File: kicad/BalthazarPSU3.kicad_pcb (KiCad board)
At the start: 2 copper layers, 85.9 x 25.4 mm, 84 parts, among them IC1 BQ24193, J1 AudioIN, J2 USB_C_Receptacle_USB2.0, J3 5-15V / 3-5A, J4 AudioOUT, J7 uC host, J8 5V 3A, J9 12V 2A, Q1 IRF7404, Q2 BSS138, Q3 BSS138, U1 PAM8403-SOP16, U3 TPS63020, U4 LM2623

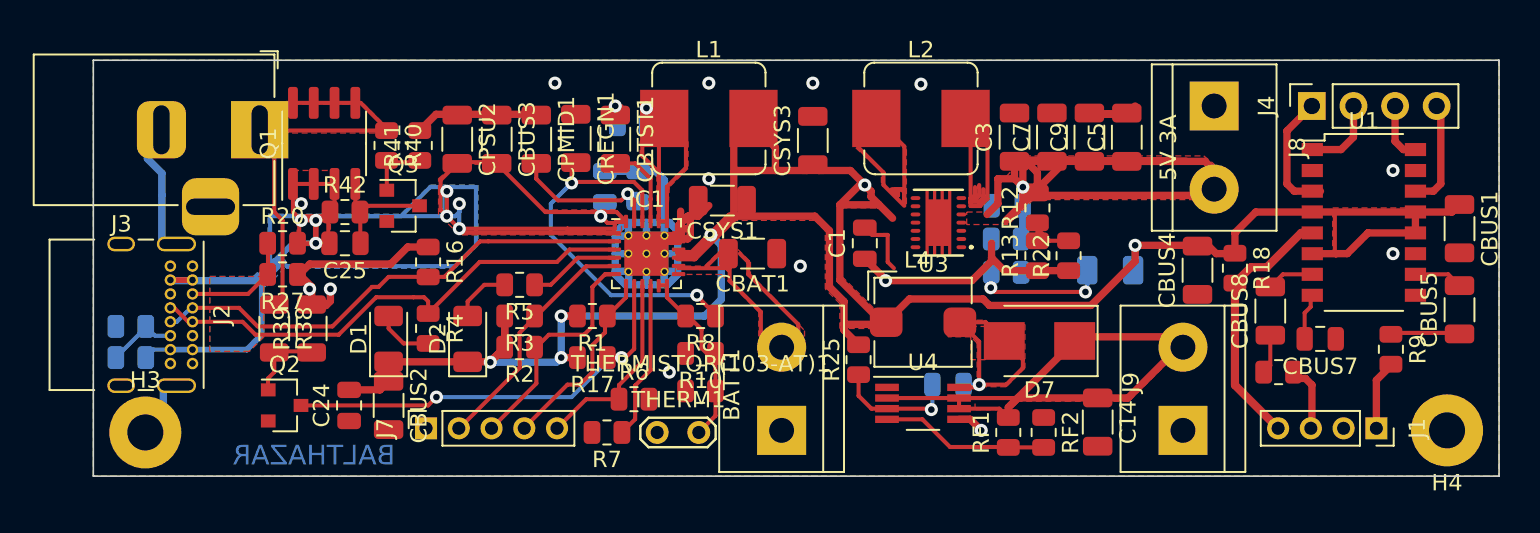
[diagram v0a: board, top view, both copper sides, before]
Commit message: Adding info fix #9
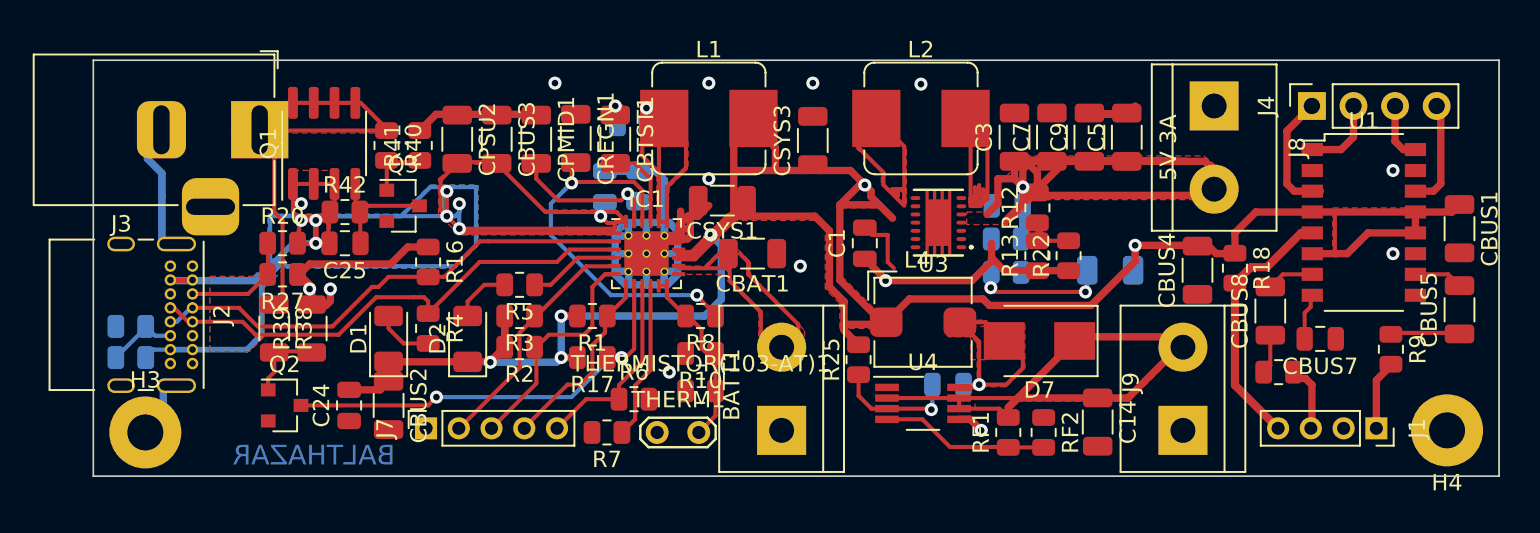
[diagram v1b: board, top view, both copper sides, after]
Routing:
- added copper zone on In1.Cu, net PGND
- added copper zone on In2.Cu, net PGND
- removed copper zone on B.Cu, net PGND
- removed copper zone on F.Cu, net PGND
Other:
- copper layers 2 -> 4
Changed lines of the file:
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@@
   )
   (paper "A4")
+  (title_block
+    (title "Balthazar PSU")
+    (date "2022-10-11")
+    (rev "v02")
+    (company "Balthazar Foundation ")
+    (comment 1 "License: CERN-OHL-S")
+  )
   (layers
     (0 "F.Cu" signal)
+    (1 "In1.Cu" power)
+    (2 "In2.Cu" power)
     (31 "B.Cu" signal)
     (32 "B.Adhes" user "B.Adhesive")
@@
   )
   (setup
+    (stackup
+      (layer "F.SilkS" (type "Top Silk Screen"))
+      (layer "F.Paste" (type "Top Solder Paste"))
+      (layer "F.Mask" (type "Top Solder Mask") (thickness 0.01))
+      (layer "F.Cu" (type "copper") (thickness 0.035))
+      (layer "dielectric 1" (type "prepreg") (thickness 0.1) (material "FR4") (epsilon_r 4.5) (loss_tangent 0.02))
+      (layer "In1.Cu" (type "copper") (thickness 0.035))
+      (layer "dielectric 2" (type "core") (thickness 1.24) (material "FR4") (epsilon_r 4.5) (loss_tangent 0.02))
+      (layer "In2.Cu" (type "copper") (thickness 0.035))
+      (layer "dielectric 3" (type "prepreg") (thickness 0.1) (material "FR4") (epsilon_r 4.5) (loss_tangent 0.02))
+      (layer "B.Cu" (type "copper") (thickness 0.035))
+      (layer "B.Mask" (type "Bottom Solder Mask") (thickness 0.01))
+      (layer "B.Paste" (type "Bottom Solder Paste"))
+      (layer "B.SilkS" (type "Bottom Silk Screen"))
+      (copper_finish "None")
+      (dielectric_constraints no)
+    )
     (pad_to_mask_clearance 0)
     (pcbplotparams
@@
     )
   )
-  (zone (net 1) (net_name "PGND") (layer "F.Cu") (hatch edge 0.508)
-    (connect_pads yes (clearance 0.508))
-    (min_thickness 0.254) (filled_areas_thickness no)
-    (fill yes (thermal_gap 0.25) (thermal_bridge_width 0.508))
-    (polygon
-      (pts
-        (xy 186.69 83.439)
-        (xy 100.838 83.439)
-        (xy 100.838 58.039)
-        (xy 186.69 58.039)
-      )
-    )
-  )
   (zone locked (net 5) (net_name "VBUS") (layer "F.Cu") (hatch edge 0.508)
     (connect_pads yes (clearance 0.508))
@@
     )
   )
+  (zone (net 1) (net_name "PGND") (layer "In1.Cu") (hatch edge 0.508)
+    (connect_pads yes (clearance 0.508))
+    (min_thickness 0.254) (filled_areas_thickness no)
+    (fill yes (thermal_gap 0.25) (thermal_bridge_width 0.508))
+    (polygon
+      (pts
+        (xy 186.69 83.439)
+        (xy 100.838 83.439)
+        (xy 100.838 58.039)
+        (xy 186.69 58.039)
+      )
+    )
+  )
+  (zone (net 1) (net_name "PGND") (layer "In2.Cu") (hatch edge 0.508)
+    (connect_pads yes (clearance 0.508))
+    (min_thickness 0.254) (filled_areas_thickness no)
+    (fill yes (thermal_gap 0.25) (thermal_bridge_width 0.508))
+    (polygon
+      (pts
+        (xy 186.69 83.439)
+        (xy 100.838 83.439)
+        (xy 100.838 58.039)
+        (xy 186.69 58.039)
+      )
+    )
+  )
   (zone locked (net 5) (net_name "VBUS") (layer "B.Cu") (name "VBUSBOT") (hatch full 0.508)
     (priority 3)
@@
       )
     )
-  )
-  (zone (net 1) (net_name "PGND") (layer "B.Cu") (hatch edge 0.508)
-    (connect_pads yes (clearance 0.508))
-    (min_thickness 0.254) (filled_areas_thickness no)
-    (fill yes (thermal_gap 0.25) (thermal_bridge_width 0.508))
-    (polygon
-      (pts
-        (xy 186.69 83.439)
-        (xy 100.838 83.439)
-        (xy 100.838 58.039)
-        (xy 186.69 58.039)
-      )
-    )

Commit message: Removing all routed signal loops
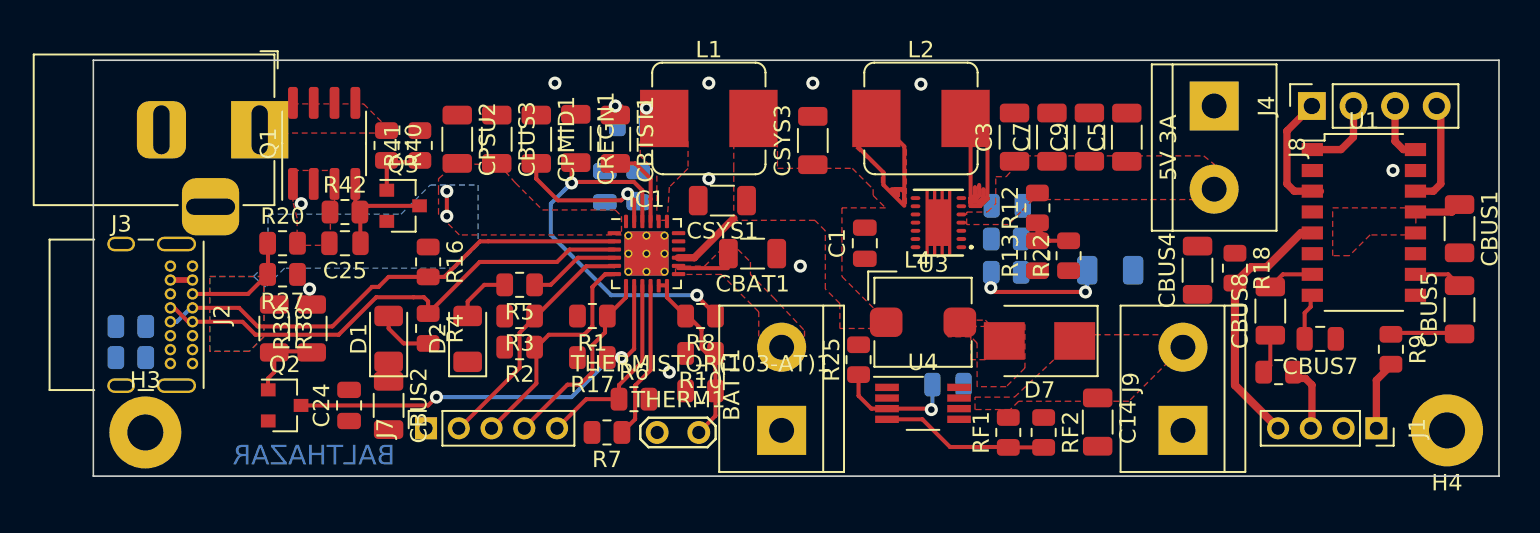
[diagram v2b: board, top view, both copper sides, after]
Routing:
- net VSYS: track 160.4 -> 7.19 mm, vias 6 -> 0
- net VBUS: track 133.5 -> 2.87 mm, vias 9 -> 3
- net PGND: track 117.1 -> 0.21 mm, vias 13 -> 9
- net 5V: track 62.8 -> 0.00 mm, vias 1 -> 0
- net 12V: track 39.9 -> 0.11 mm
- net VPSU: track 30.0 -> 0.00 mm
- net Net-(IC1-SW): track 17.5 -> 1.04 mm
- net Net-(BATT1-Pin_2): track 18.3 -> 3.03 mm
- net Net-(D7-A): track 15.3 -> 0.16 mm, vias 1 -> 0
- net Net-(J2-CC2): track 4.40 -> 0.00 mm

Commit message: Routing all signals fix #11 fix #7
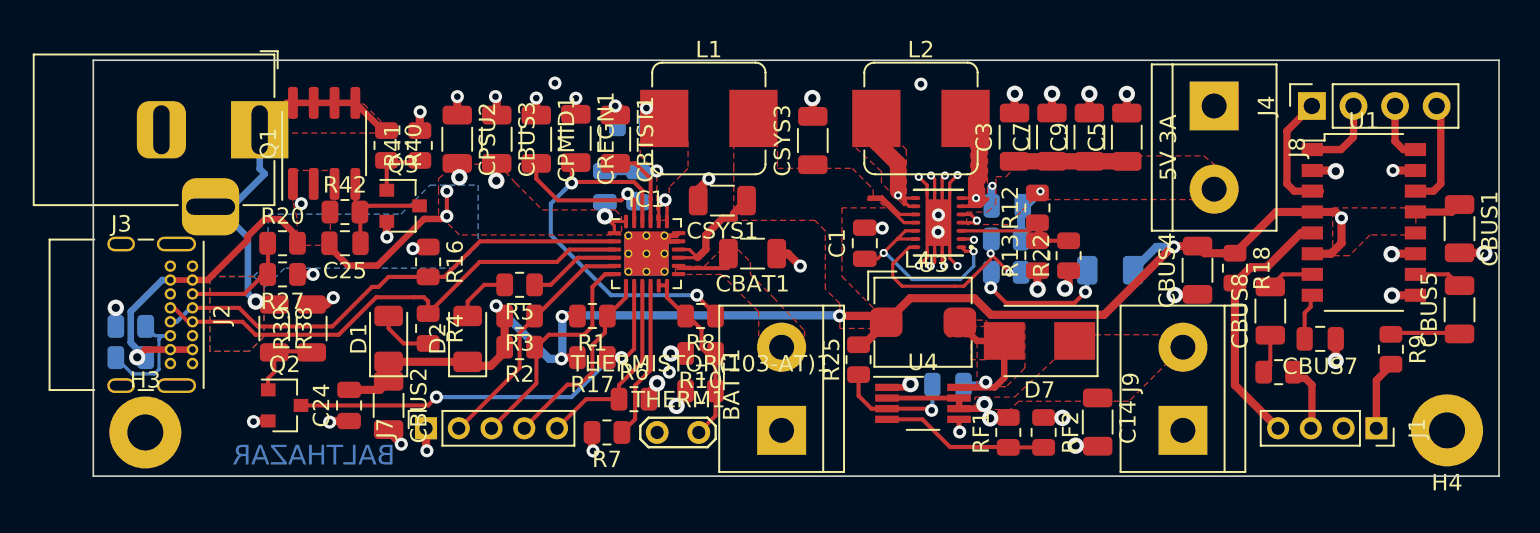
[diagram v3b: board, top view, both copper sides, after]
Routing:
- net VSYS: track 7.19 -> 103.0 mm, vias 0 -> 6
- net PGND: track 0.21 -> 64.2 mm, vias 9 -> 55
- net VBUS: track 2.87 -> 36.9 mm, vias 3 -> 7
- net VPSU: track 0.00 -> 24.5 mm, vias 0 -> 1
- net Net-(U3-EN): track 0.00 -> 13.2 mm, vias 0 -> 2
- net Net-(U3-PG): track 0.00 -> 13.1 mm, vias 0 -> 2
- net 5V: track 0.00 -> 12.5 mm, vias 0 -> 2
- net Net-(D7-A): track 0.16 -> 9.92 mm, vias 0 -> 1
- net 12V: track 0.11 -> 7.86 mm, vias 0 -> 2
- net Net-(J2-CC2): track 0.00 -> 7.55 mm
- net Net-(U3-L1): track 15.0 -> 10.1 mm, vias 0 -> 1
- net Net-(R13-Pad2): track 3.30 -> 8.15 mm
- net Net-(U3-L2): track 15.4 -> 12.5 mm, vias 0 -> 1
- net Net-(IC1-SW): track 1.04 -> 3.88 mm, vias 1 -> 2
- net Net-(D4-C): track 8.21 -> 8.76 mm
